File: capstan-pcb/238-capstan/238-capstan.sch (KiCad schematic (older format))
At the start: 53 parts, among them CN1 CN1, IC1 BA6303F, IC2 4013, IC3 BA6411, J1 0, J2 0

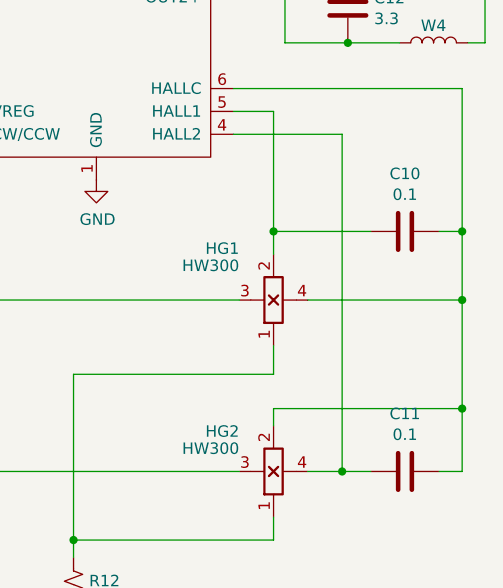
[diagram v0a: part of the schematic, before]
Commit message: Capstan pcb v2024-08-04
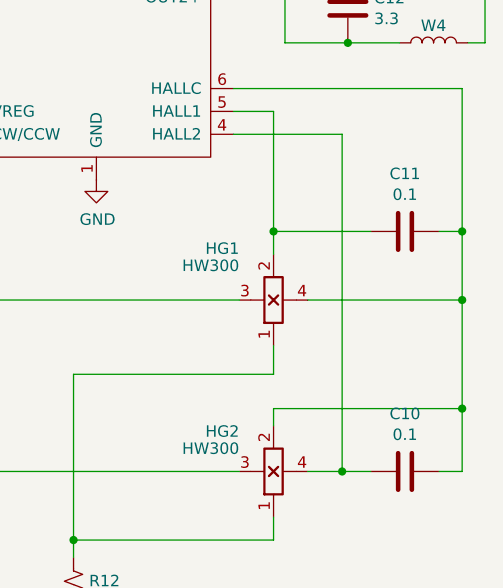
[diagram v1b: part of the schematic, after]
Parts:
- renumbered C11 to C10, C10 to C11
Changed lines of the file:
@@
 $EndComp
 $Comp
-L Device:C C11
+L Device:C C10
 U 1 1 66AE44D5
 P 9225 5175
-F 0 "C11" V 9477 5175 50  0000 C CNN
+F 0 "C10" V 9477 5175 50  0000 C CNN
 F 1 "0.1" V 9386 5175 50  0000 C CNN
 F 2 "Capacitor_SMD:C_1206_3216Metric_Pad1.33x1.80mm_HandSolder" H 9263 5025 50  0001 C CNN
@@
 $EndComp
 $Comp
-L Device:C C10
+L Device:C C11
 U 1 1 66AE3DF6
 P 9225 4125
-F 0 "C10" V 9477 4125 50  0000 C CNN
+F 0 "C11" V 9477 4125 50  0000 C CNN
 F 1 "0.1" V 9386 4125 50  0000 C CNN
 F 2 "Capacitor_SMD:C_1206_3216Metric_Pad1.33x1.80mm_HandSolder" H 9263 3975 50  0001 C CNN
